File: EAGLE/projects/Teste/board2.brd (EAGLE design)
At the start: 92.6 x 71.1 mm, 21 parts, among them IC1 317T, IC2 7805T

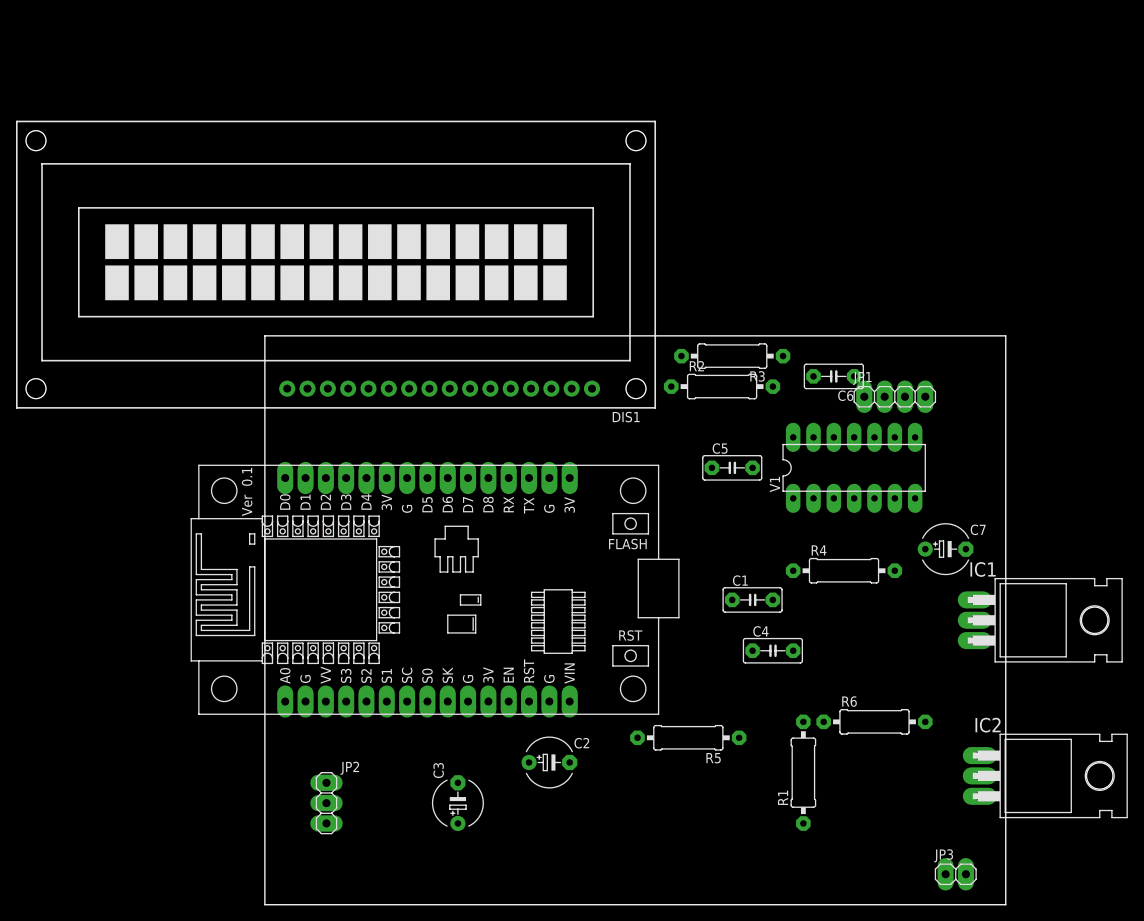
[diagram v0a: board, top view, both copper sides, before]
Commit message: roteamento
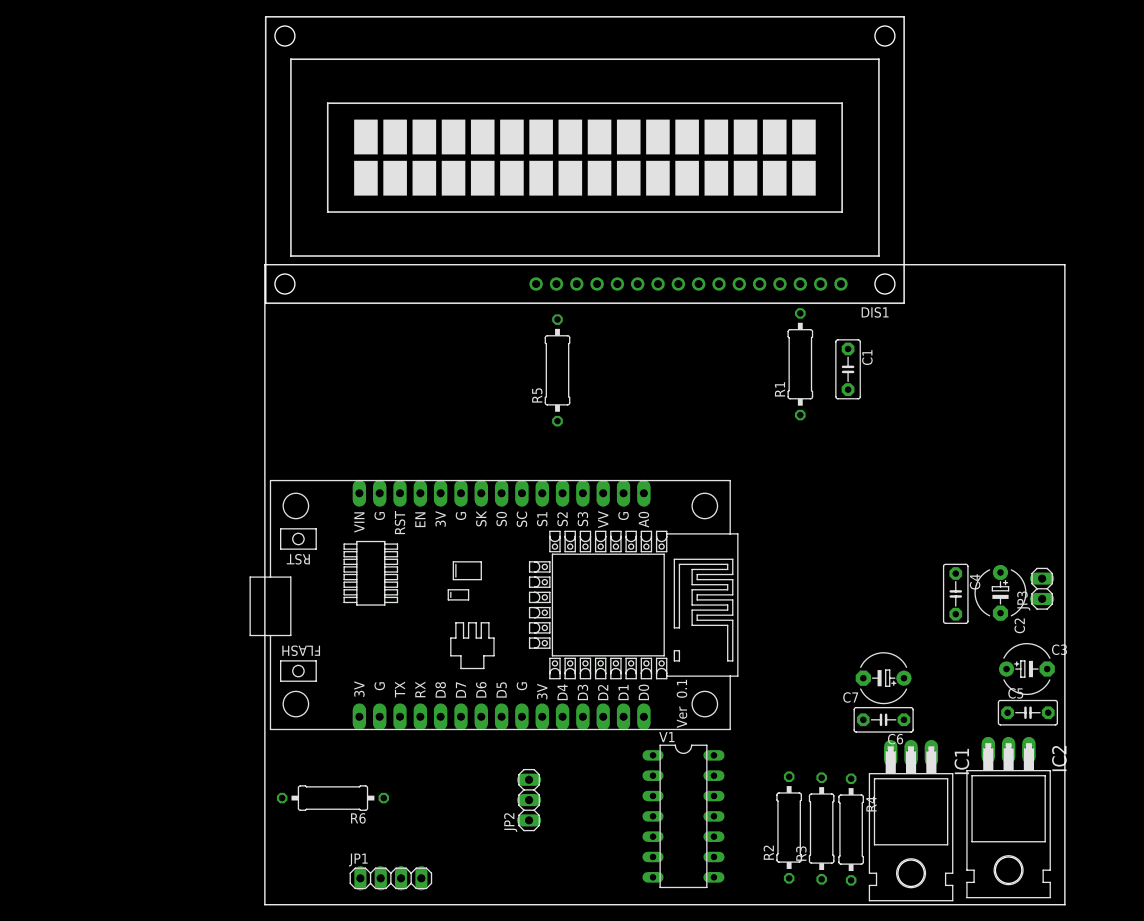
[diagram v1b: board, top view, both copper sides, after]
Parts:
- C1, C4, C5, C6: value (none) -> 100nF
- C2: value (none) -> 47uF
- C3, C7: value (none) -> 10nF
- R1: value (none) -> 2K2
- R2, R3: value (none) -> 120
- R4: value (none) -> 390
- R5: value (none) -> 33
- R6: value (none) -> 10K
- moved JP1 87.1 mm to (15.7, 3.30)
- moved C3 73.1 mm to (95.2, 29.5), turned to 0 degrees
- moved R6 68.4 mm to (8.51, 13.3), turned to 180 degrees
- moved C2 60.2 mm to (91.9, 39.0), turned to 270 degrees
- moved R3 60.1 mm to (69.6, 9.53), turned to 90 degrees
- moved R2 55.8 mm to (65.5, 9.65), turned to 90 degrees
- moved R1 51.1 mm to (66.9, 67.6)
- moved R5 48.8 mm to (36.6, 66.8), turned to 90 degrees
- moved V1 48.5 mm to (52.3, 11.0), turned to 270 degrees
- moved C5 48.0 mm to (95.4, 24.0)
- moved C6 43.4 mm to (77.3, 23.1)
- moved JP3 37.3 mm to (97.2, 39.5), turned to 90 degrees
- moved DIS1 33.8 mm to (40.0, 93.1)
- moved R4 32.4 mm to (73.3, 9.40), turned to 270 degrees
- moved IC1 32.4 mm to (80.8, 8.76), turned to 180 degrees
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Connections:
- net +5V: now also U$1.15
- net MOTOR: now also U$1.28; no longer U$1.4
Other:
- board size 92.6 x 71.1 mm -> 100 x 80 mm
